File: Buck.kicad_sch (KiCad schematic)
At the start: 15 parts, among them J1 IN, J2 OUT, J3 Measure, U1 LT1936

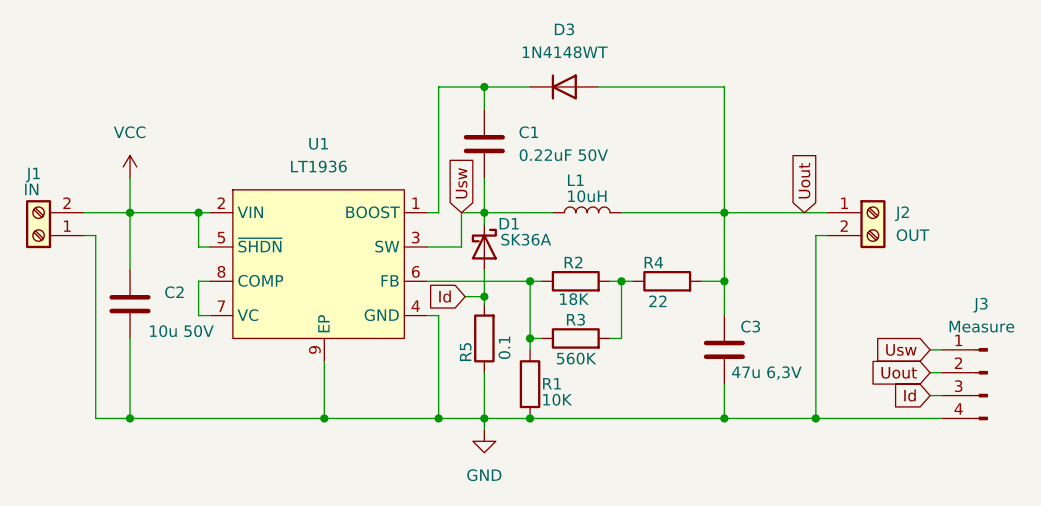
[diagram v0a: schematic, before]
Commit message: small tweaks trace layout
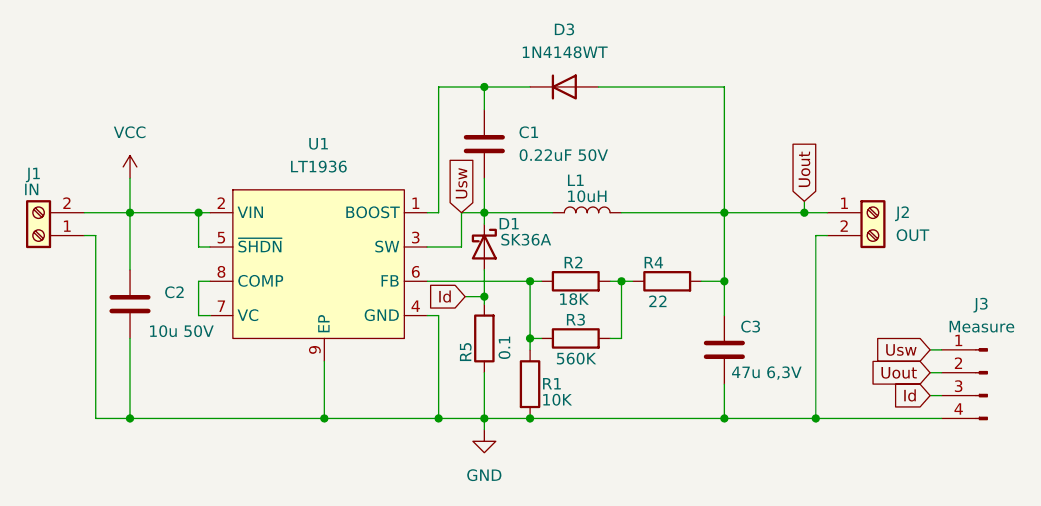
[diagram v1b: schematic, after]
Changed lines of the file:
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@@
 	(paper "A4")
 	(junction
+		(at 137.16 87.63)
+		(diameter 0)
+		(color 0 0 0 0)
+	)
+	(junction
 		(at 62.23 87.63)
 		(diameter 0)
@@
 	(wire
 		(pts
+			(xy 137.16 87.63) (xy 139.7 87.63)
+		)
+		(stroke
+			(width 0)
+			(type default)
+		)
+	)
+	(wire
+		(pts
 			(xy 83.82 104.14) (xy 83.82 110.49)
 		)
@@
 	(wire
 		(pts
-			(xy 128.27 87.63) (xy 139.7 87.63)
+			(xy 128.27 87.63) (xy 137.16 87.63)
 		)
 		(stroke
@@
 		(pts
 			(xy 101.6 93.98) (xy 101.6 96.9578)
+		)
+		(stroke
+			(width 0)
+			(type default)
+		)
+	)
+	(wire
+		(pts
+			(xy 137.16 86.36) (xy 137.16 87.63)
 		)
 		(stroke
@@
 	(global_label "Uout"
 		(shape input)
-		(at 137.16 87.63 90)
+		(at 137.16 86.36 90)
 		(fields_autoplaced yes)
 		(effects
@@
 		)
 		(property "Intersheetrefs" "${INTERSHEET_REFS}"
-			(at 137.16 80.2906 90)
+			(at 137.16 79.0206 90)
 			(effects
 				(font
